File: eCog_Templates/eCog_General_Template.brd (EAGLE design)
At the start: 48 x 28 mm, 10 parts

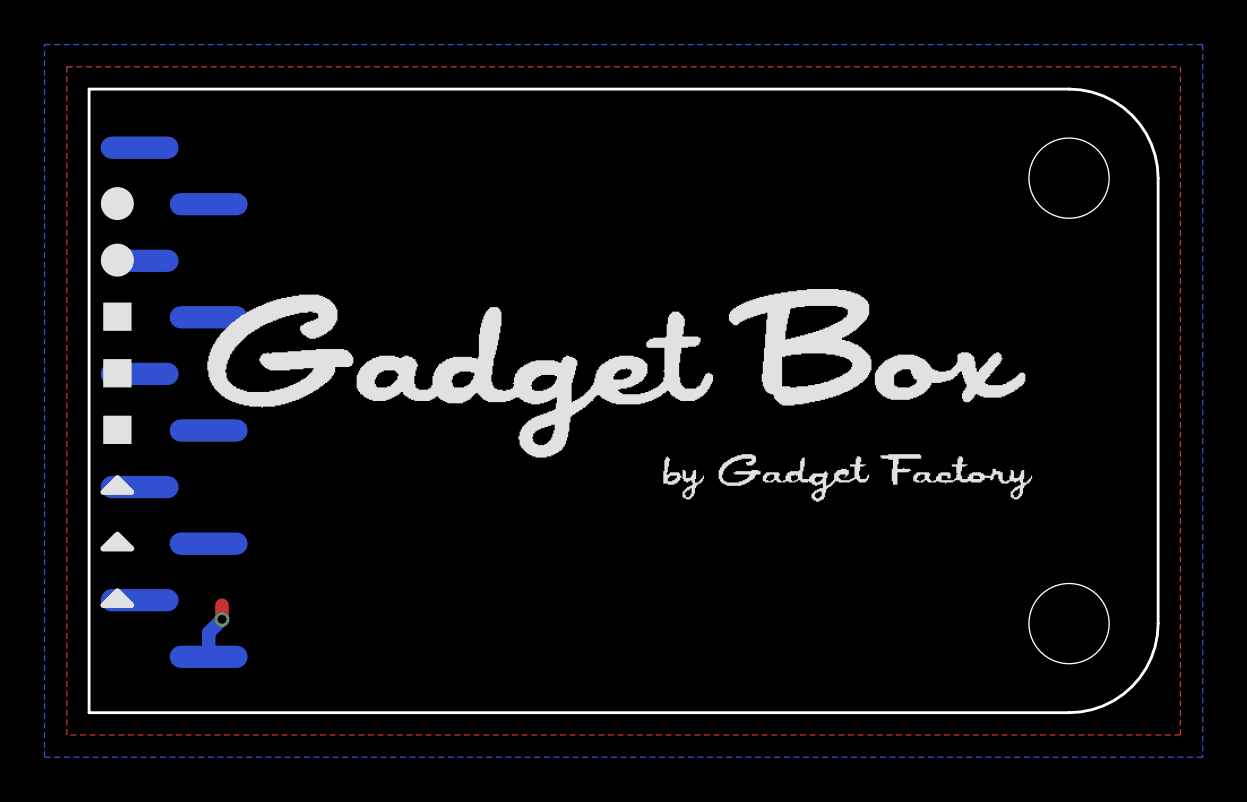
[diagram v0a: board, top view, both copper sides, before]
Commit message: All the 2.0 updates
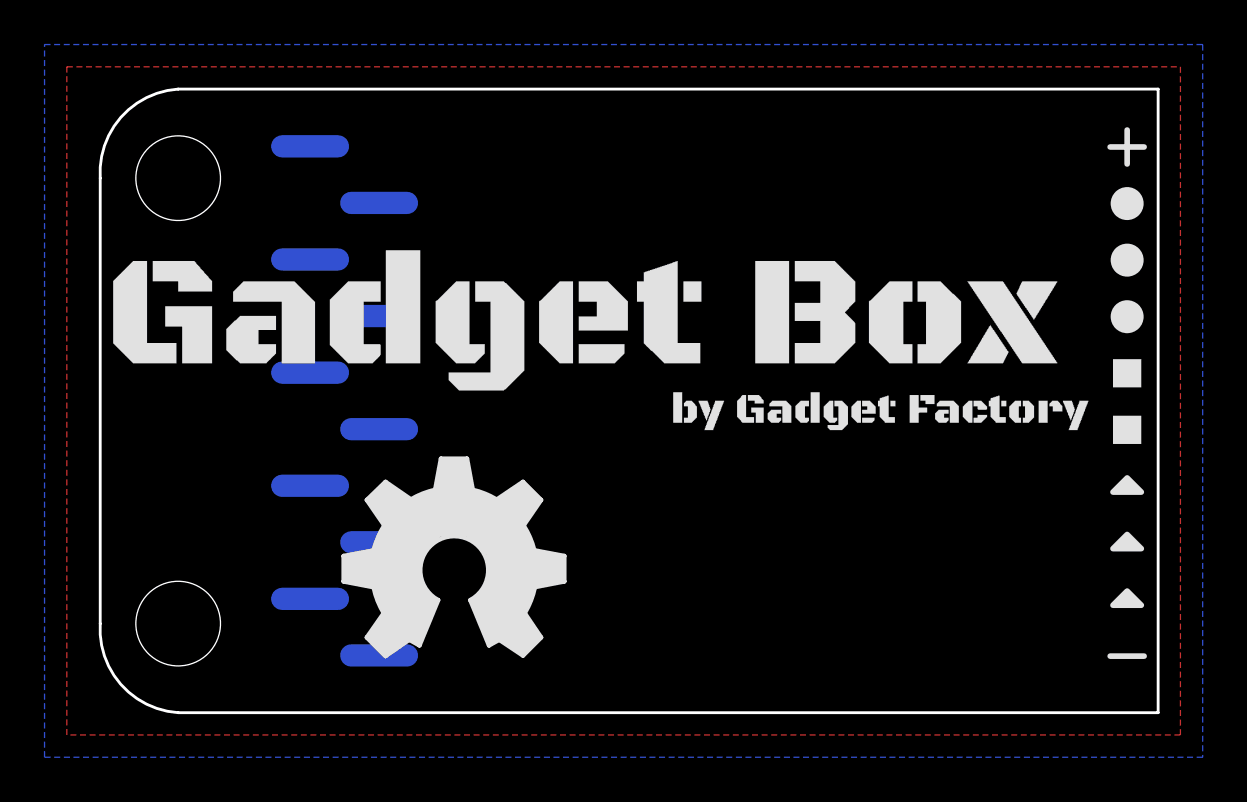
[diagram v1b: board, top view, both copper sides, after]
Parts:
- added U$10: (no value), ohw-logo:OSHW_FILLX350_NOTEXT
- U$4: device eCogs:LEGEND_PWM -> eCogs:LEGEND_DIO
- moved U$2 45.3 mm to (46.6, 22.9)
- moved U$3 45.3 mm to (46.6, 20.3)
- moved U$4 45.3 mm to (46.6, 17.8)
- moved U$5 45.3 mm to (46.6, 15.2)
- moved U$6 45.3 mm to (46.6, 12.7)
- moved U$7 45.3 mm to (46.6, 10.2)
- moved U$8 45.3 mm to (46.6, 7.62)
- moved U$9 45.3 mm to (46.6, 5.08)
- moved U$1 2.80 mm to (22.4, 17.4)
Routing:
- net 3V3: track 2.56 -> 0.00 mm, vias 1 -> 0
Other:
- board size 48 x 28 mm -> 47.5 x 28 mm
- board text added: "0"
- board text added: "1"
- board text added: "2"
- board text added: "3"
- board text added: "4"
- board text added: "5"
- board text added: "6"
- board text added: "7"
- board text added: "ecog100 v2.0"
- board text removed: "G0<>"
- board text removed: "G1<>"
- board text removed: "G2<>"
- board text removed: "G3<>"
- board text removed: "G4<>"
- board text removed: "G5<>"
- board text removed: "G6<>"
- board text removed: "G7<>"
- board text removed: "ecog100 v1.0"
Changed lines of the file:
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@@
 <plain>
 <text x="37.559" y="18.415" size="0.8128" layer="22" font="vector" rot="MR0">ecog100.GadgetFactory.net</text>
-<text x="39.702" y="2.159" size="1.016" layer="22" font="vector" rot="MR0">ecog100 v1.0</text>
+<text x="39.702" y="2.159" size="1.016" layer="22" font="vector" rot="MR0">ecog100 v2.0</text>
 <text x="39.702" y="3.429" size="1.016" layer="22" font="vector" rot="MR0">Project Name</text>
 <text x="39.702" y="4.699" size="1.016" layer="22" font="vector" rot="MR0">eCogs</text>
-<text x="11.335" y="19.812" size="1.016" layer="22" font="vector" rot="MR0">G1&lt;&gt;</text>
-<text x="11.335" y="17.272" size="1.016" layer="22" font="vector" rot="MR0">G2&lt;&gt;</text>
-<text x="11.335" y="14.732" size="1.016" layer="22" font="vector" rot="MR0">G3&lt;&gt;</text>
-<text x="11.335" y="12.192" size="1.016" layer="22" font="vector" rot="MR0">G4&lt;&gt;</text>
-<text x="11.335" y="9.652" size="1.016" layer="22" font="vector" rot="MR0">G5&lt;&gt;</text>
-<text x="11.335" y="7.112" size="1.016" layer="22" font="vector" rot="MR0">G6&lt;&gt;</text>
-<text x="11.335" y="4.572" size="1.016" layer="22" font="vector" rot="MR0">G7&lt;&gt;</text>
-<text x="11.335" y="22.352" size="1.016" layer="22" font="vector" rot="MR0">G0&lt;&gt;</text>
+<text x="15.335" y="8.128" size="1.016" layer="22" font="vector" rot="MR180">1</text>
+<text x="15.335" y="10.668" size="1.016" layer="22" font="vector" rot="MR180">2</text>
+<text x="15.335" y="13.208" size="1.016" layer="22" font="vector" rot="MR180">3</text>
+<text x="15.335" y="15.748" size="1.016" layer="22" font="vector" rot="MR180">4</text>
+<text x="15.335" y="18.288" size="1.016" layer="22" font="vector" rot="MR180">5</text>
+<text x="15.335" y="20.828" size="1.016" layer="22" font="vector" rot="MR180">6</text>
+<text x="15.335" y="23.368" size="1.016" layer="22" font="vector" rot="MR180">7</text>
+<text x="15.335" y="5.588" size="1.016" layer="22" font="vector" rot="MR180">0</text>
 <text x="33.782" y="17.526" size="0.6096" layer="22" font="vector" rot="MR0">Copyright 2016</text>
 <text x="35.512" y="16.637" size="0.6096" layer="22" font="vector" rot="MR0">Gadget Factory, LLC</text>
-<text x="11.335" y="2.032" size="1.016" layer="22" font="vector" rot="MR0">3.3V</text>
-<text x="11.335" y="24.892" size="1.016" layer="22" font="vector" rot="MR0">GND</text>
+<text x="15.335" y="25.908" size="1.016" layer="22" font="vector" rot="MR180">3.3V</text>
+<text x="15.335" y="3.048" size="1.016" layer="22" font="vector" rot="MR180">GND</text>
+<wire x1="45.847" y1="25.4" x2="47.371" y2="25.4" width="0.254" layer="21"/>
+<wire x1="46.609" y1="26.162" x2="46.609" y2="24.638" width="0.254" layer="21"/>
+<wire x1="45.847" y1="2.54" x2="47.371" y2="2.54" width="0.254" layer="21"/>
 </plain>
 <attributes>
@@
 </autorouter>
 <elements>
-<element name="ECOG" library="eCogs" package="ECOG_GENERAL_SMD" value="ECOG_GENERAL_ROWECOG_GENERAL_SMD" x="0" y="0" smashed="yes"/>
-<element name="U$1" library="GadgetFactory" package="GADGETBOX_TEXT" value="" x="24.13" y="15.24"/>
-<element name="U$2" library="eCogs" package="LEGEND_DIO" value="" x="1.27" y="22.86"/>
-<element name="U$3" library="eCogs" package="LEGEND_DIO" value="" x="1.27" y="20.32"/>
-<element name="U$4" library="eCogs" package="LEGEND_PWM" value="" x="1.27" y="17.78"/>
-<element name="U$5" library="eCogs" package="LEGEND_PWM" value="" x="1.27" y="15.24"/>
-<element name="U$6" library="eCogs" package="LEGEND_PWM" value="" x="1.27" y="12.7"/>
-<element name="U$7" library="eCogs" package="LEGEND_ANALOG" value="" x="1.27" y="10.16"/>
-<element name="U$8" library="eCogs" package="LEGEND_ANALOG" value="" x="1.27" y="7.62"/>
-<element name="U$9" library="eCogs" package="LEGEND_ANALOG" value="" x="1.27" y="5.08"/>
+<element name="ECOG" library="eCogs" package="ECOG_GENERAL_SMD" value="ECOG_GENERAL_ROWECOG_GENERAL_SMD" x="0" y="0" smashed="yes">
+<attribute name="DIGIKEY" value="S1013EC-10-ND" x="0" y="0" size="1.778" layer="27" display="off"/>
+</element>
+<element name="U$2" library="eCogs" package="LEGEND_DIO" value="" x="46.609" y="22.86"/>
+<element name="U$3" library="eCogs" package="LEGEND_DIO" value="" x="46.609" y="20.32"/>
+<element name="U$5" library="eCogs" package="LEGEND_PWM" value="" x="46.609" y="15.24"/>
+<element name="U$6" library="eCogs" package="LEGEND_PWM" value="" x="46.609" y="12.7"/>
+<element name="U$7" library="eCogs" package="LEGEND_ANALOG" value="" x="46.609" y="10.16"/>
+<element name="U$8" library="eCogs" package="LEGEND_ANALOG" value="" x="46.609" y="7.62"/>
+<element name="U$9" library="eCogs" package="LEGEND_ANALOG" value="" x="46.609" y="5.08"/>
+<element name="U$1" library="GadgetFactory" package="GADGETBOX_TEXT" value="" x="22.352" y="17.399"/>
+<element name="U$10" library="ohw-logo" package="OSHW_FILLX350_NOTEXT" value="" x="11.43" y="2.54"/>
+<element name="U$4" library="eCogs" package="LEGEND_DIO" value="" x="46.609" y="17.78"/>
 </elements>
 <signals>
@@
 <vertex x="-1" y="-1"/>
 </polygon>
-<wire x1="5.3694" y1="2.51" x2="5.3694" y2="3.5914" width="0.6096" layer="16"/>
-<wire x1="5.3694" y1="3.5914" x2="5.969" y2="4.191" width="0.6096" layer="16"/>
-<via x="5.969" y="4.191" extent="1-16" drill="0.381"/>
-<wire x1="5.969" y1="4.191" x2="5.969" y2="4.826" width="0.6096" layer="1"/>
 </signal>
 </signals>
